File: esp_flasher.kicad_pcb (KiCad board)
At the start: 2 copper layers, 43 x 20 mm, 29 parts, among them J1 USB_B_Micro, J2 Conn_01x06, J3 boot btn, J4 en btn, Q1 S8050, Q2 S8050, U1 ZLDO1117QG33TA_SOT223, U2 CP2102N-A01-GQFN28

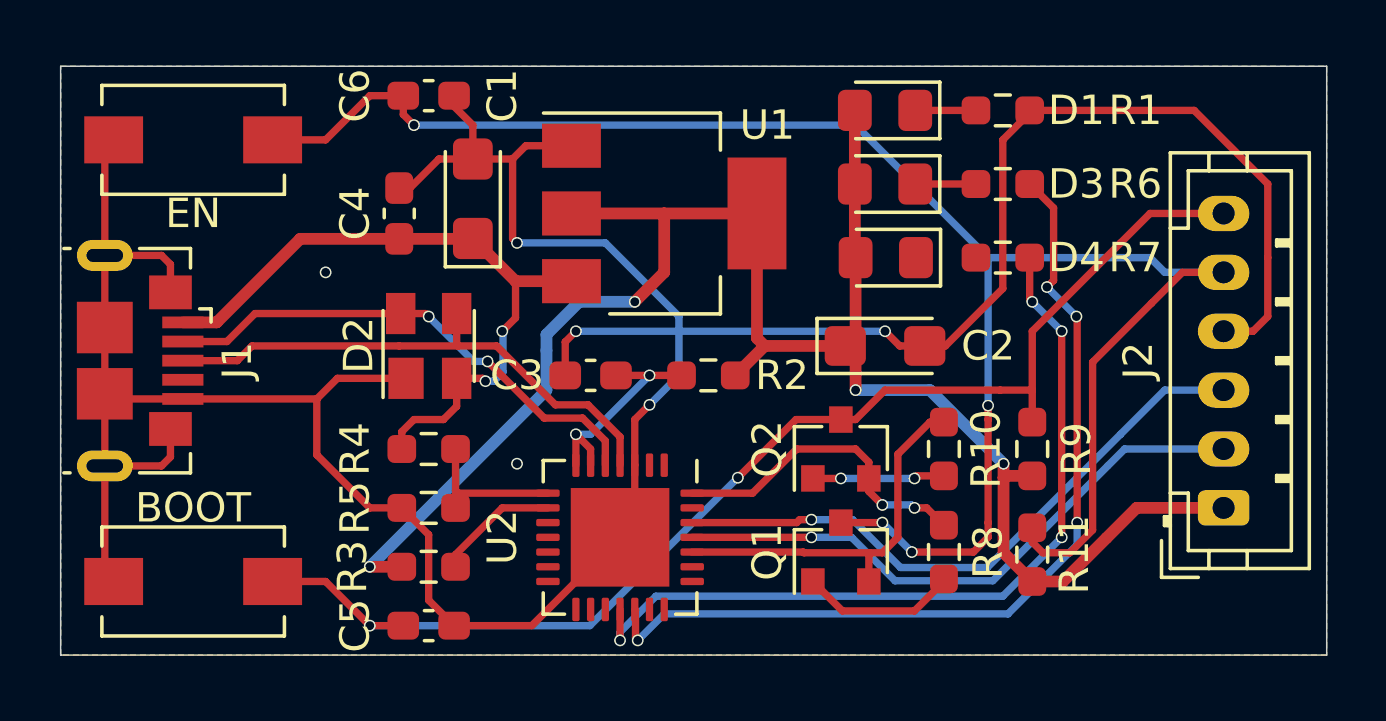
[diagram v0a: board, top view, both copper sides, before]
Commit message: 2021-07-20 2
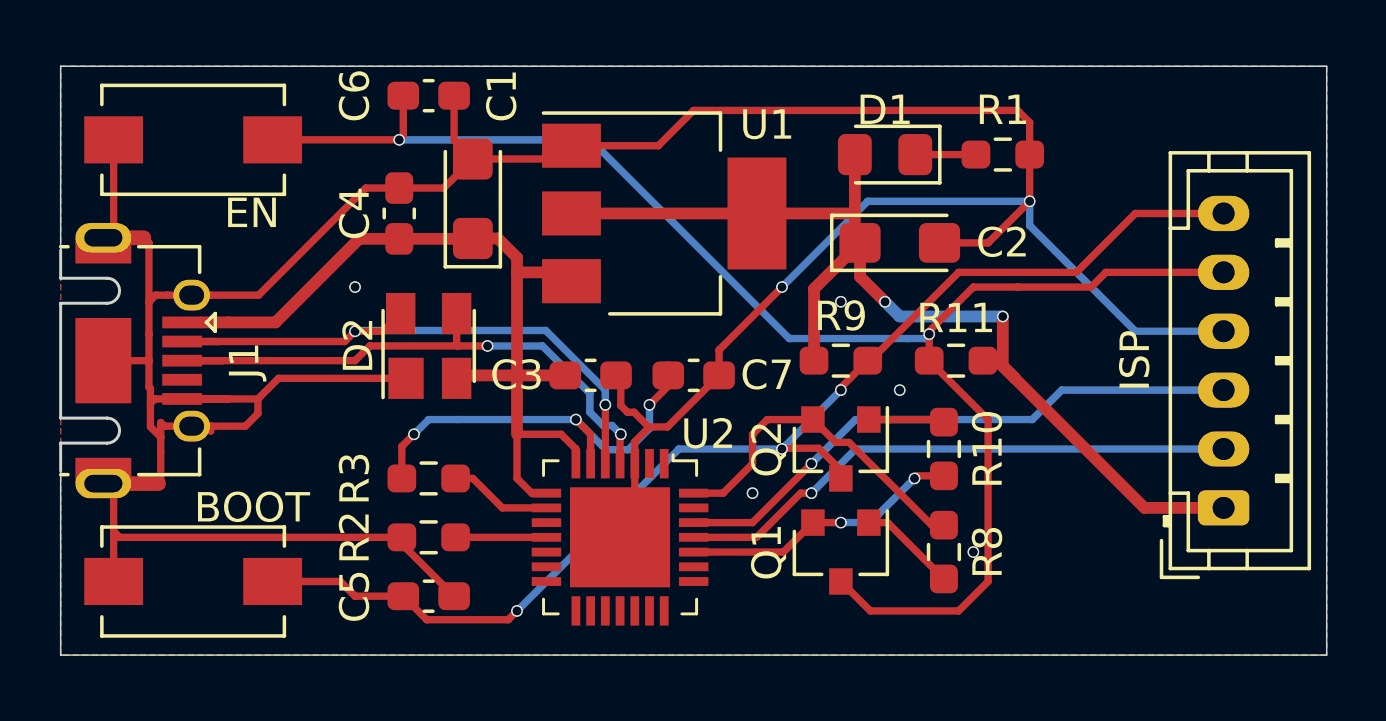
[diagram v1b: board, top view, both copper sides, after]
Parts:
- removed D3, D4: led, LED_SMD:LED_0805_2012Metric_Pad1.15x1.40mm_HandSolder
- removed R4: 22.1k, Resistor_SMD:R_0603_1608Metric_Pad0.98x0.95mm_HandSolder
- removed R5: 47.5k, Resistor_SMD:R_0603_1608Metric_Pad0.98x0.95mm_HandSolder
- removed R6, R7: 470, Resistor_SMD:R_0603_1608Metric_Pad0.98x0.95mm_HandSolder
- added C7: 0.1u, Capacitor_SMD:C_0603_1608Metric_Pad1.08x0.95mm_HandSolder, F.Cu at (21.5, 10.5)
- J1: footprint Connector_USB:USB_Micro-B_GCT_USB3076-30-A -> Connector_USB:USB_Micro-AB_Molex_47590-0001
- R2: value 0 -> NC
- R3: value 1k -> 4.7k
- U2: value CP2102N-A01-GQFN28 -> CP2102-GMR_NRND; footprint Package_DFN_QFN:QFN-28-1EP_5x5mm_P0.5mm_EP3.35x3.35mm -> digikey-footprints:VFQFN-28-1EP_5x5mm
- moved R2 11.0 mm to (12.5, 16.0)
- moved R9 7.16 mm to (26.5, 10.0), turned to 180 degrees
- moved R11 7.08 mm to (30.4, 10.0), turned to 0 degrees
- moved C2 3.54 mm to (28.5, 6.00)
- moved R3 3.00 mm to (12.5, 14.0), turned to 180 degrees
- moved D1 1.50 mm to (28.0, 3.00)
- moved R1 1.50 mm to (32.0, 3.00)
- moved J1 1.25 mm to (1.45, 10.0)
- moved C5 1.00 mm to (12.5, 18.0)
- turned C3 to 0 degrees
- turned Q1 to 270 degrees
- turned Q2 to 270 degrees
- turned R10 to 90 degrees
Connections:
- C3 pad 1: Net-(C3-Pad1) -> +5V
- R2 pad 1: Net-(C3-Pad1) -> Earth
- R2 pad 2: +3V3 -> Net-(R2-Pad2)
- R3 pad 1: +3V3 -> Net-(R3-Pad1)
- R3 pad 2: Net-(R3-Pad2) -> Net-(C7-Pad1)
- U2 pad 11: Net-(U2-Pad11) -> Net-(R2-Pad2)
- U2 pad 6: Net-(C3-Pad1) -> Net-(C7-Pad1)
- U2 pad 7: Net-(C3-Pad1) -> +5V
- U2 pad 8: Net-(R4-Pad2) -> +5V
- U2 pad 9: Net-(R3-Pad2) -> Net-(R3-Pad1)
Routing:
- net Net-(U2-Pad19): track 30.5 -> 0.00 mm, vias 4 -> 0
- net Net-(U2-Pad18): track 27.6 -> 0.00 mm, vias 4 -> 0
- net +3V3: track 62.2 -> 36.4 mm, vias 4 -> 2
- net Net-(C7-Pad1): track 0.00 -> 14.7 mm, vias 0 -> 3
- net EN: track 65.3 -> 52.7 mm, vias 4 -> 2
- net Net-(C3-Pad1): track 7.86 -> 0.00 mm, vias 2 -> 0
- net +5V: track 23.8 -> 30.8 mm, vias 2 -> 0
- net Earth: track 115.2 -> 121.5 mm, vias 6 -> 7
- net Net-(R4-Pad2): track 5.17 -> 0.00 mm
- net Net-(R3-Pad2): track 4.21 -> 0.00 mm
- net Net-(R3-Pad1): track 0.00 -> 3.50 mm
- net RTS: track 13.0 -> 9.57 mm, vias 0 -> 2
- net Net-(R2-Pad2): track 0.00 -> 3.09 mm
- net Net-(D2-Pad4): track 17.4 -> 20.2 mm
- net Net-(D3-Pad1): track 2.06 -> 0.00 mm
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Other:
- outline, holes or cut-outs redrawn
- board text added: "ISP"
